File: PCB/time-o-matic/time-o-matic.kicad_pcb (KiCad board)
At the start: 2 copper layers, 1 part, among them U1 ESP32-DevKitC

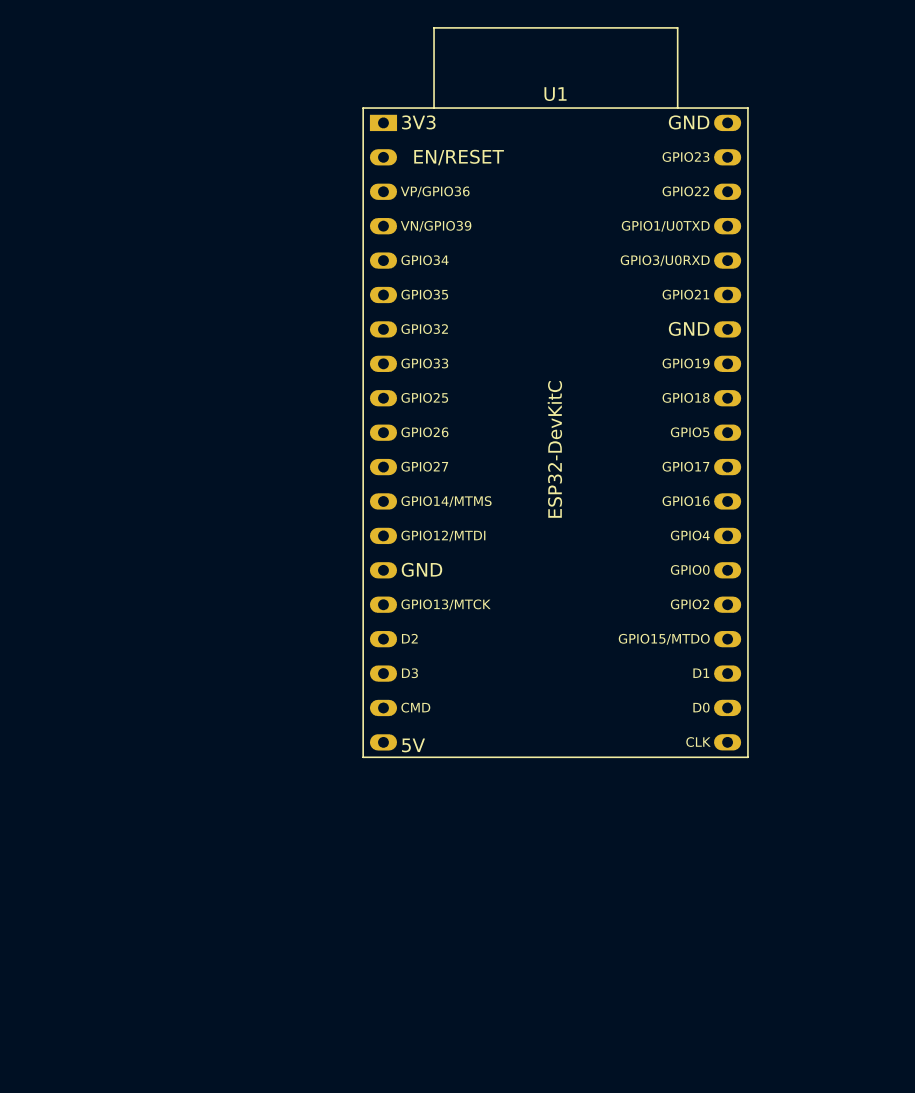
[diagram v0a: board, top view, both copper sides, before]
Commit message: W
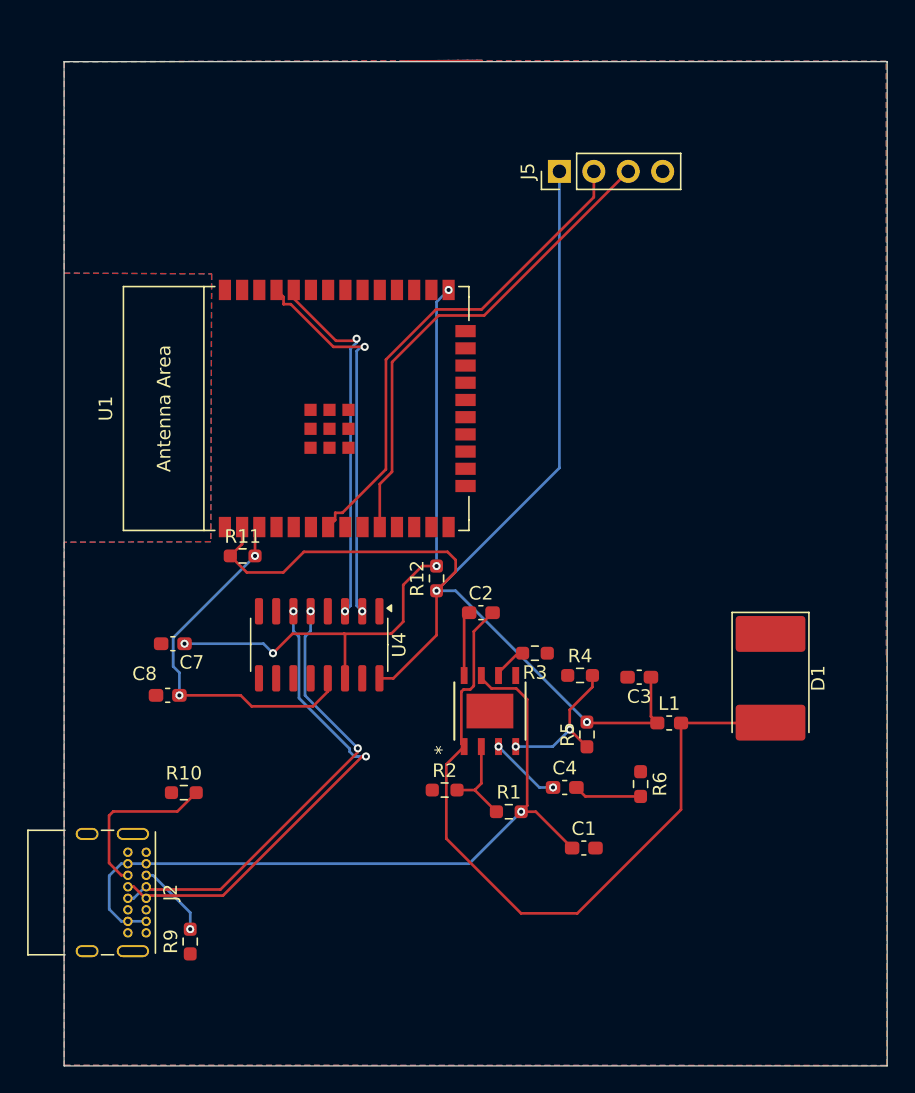
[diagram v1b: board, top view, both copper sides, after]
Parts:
- added C1: 10uF, Capacitor_SMD:C_0603_1608Metric_Pad1.08x0.95mm_HandSolder, F.Cu at (109.6, 106.0)
- added C2: 100nF, Capacitor_SMD:C_0603_1608Metric_Pad1.08x0.95mm_HandSolder, F.Cu at (102.0, 88.6)
- added C3: 22uF, Capacitor_SMD:C_0603_1608Metric_Pad1.08x0.95mm_HandSolder, F.Cu at (113.7, 93.4)
- added C4: 220pF, Capacitor_SMD:C_0603_1608Metric_Pad1.08x0.95mm_HandSolder, F.Cu at (108.2, 101.5)
- added C7: 10uF, Capacitor_SMD:C_0603_1608Metric_Pad1.08x0.95mm_HandSolder, F.Cu at (79.3, 90.9)
- added C8: 10uF, Capacitor_SMD:C_0603_1608Metric_Pad1.08x0.95mm_HandSolder, F.Cu at (78.9, 94.7)
- added D1: D_Schottky, Diode_SMD:D_3220_8050Metric_Pad2.65x5.15mm_HandSolder, F.Cu at (123.4, 93.5)
- added J2: USB_C_Receptacle_USB2.0_14P, Connector_USB:USB_C_Receptacle_GCT_USB4085, F.Cu at (77.3, 106.3)
- added J5: Display Connector, Connector_PinHeader_2.54mm:PinHeader_1x04_P2.54mm_Vertical, F.Cu at (107.8, 56.0)
- added L1: 10uH, Inductor_SMD:L_0603_1608Metric_Pad1.05x0.95mm_HandSolder, F.Cu at (115.9, 96.8)
- added R1: 100k, Resistor_SMD:R_0603_1608Metric_Pad0.98x0.95mm_HandSolder, F.Cu at (104.1, 103.3)
- added R10: 5.1k, Resistor_SMD:R_0603_1608Metric_Pad0.98x0.95mm_HandSolder, F.Cu at (80.1, 101.9)
- added R11: 10k, Resistor_SMD:R_0603_1608Metric_Pad0.98x0.95mm_HandSolder, F.Cu at (84.5, 84.4)
- added R12: 10k, Resistor_SMD:R_0603_1608Metric_Pad0.98x0.95mm_HandSolder, F.Cu at (98.8, 86.1)
- added R2: 24.9k, Resistor_SMD:R_0603_1608Metric_Pad0.98x0.95mm_HandSolder, F.Cu at (99.4, 101.7)
- added R3: 200k, Resistor_SMD:R_0603_1608Metric_Pad0.98x0.95mm_HandSolder, F.Cu at (106.0, 91.6)
- added R4: 40.2k, Resistor_SMD:R_0603_1608Metric_Pad0.98x0.95mm_HandSolder, F.Cu at (109.4, 93.2)
- added R5: 124k, Resistor_SMD:R_0603_1608Metric_Pad0.98x0.95mm_HandSolder, F.Cu at (109.9, 97.6)
- added R6: 68.1k, Resistor_SMD:R_0603_1608Metric_Pad0.98x0.95mm_HandSolder, F.Cu at (113.8, 101.3)
- added R9: 5.1k, Resistor_SMD:R_0603_1608Metric_Pad0.98x0.95mm_HandSolder, F.Cu at (80.6, 112.9)
- added U2: MP1584EN-LF-P, MP1584:SOIC8E_MPS_MNP-L, F.Cu at (102.7, 95.9)
- added U4: CH340C, Package_SO:SOIC-16_3.9x9.9mm_P1.27mm, F.Cu at (90.1, 91.0)
- U1: value ESP32-DevKitC -> ESP32-WROOM-E; footprint PCM_Espressif:ESP32-DevKitC -> PCM_Espressif:ESP32-WROOM-32E
- moved U1 21.6 mm to (90.2, 73.5), turned to 90 degrees
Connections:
- U1 pad 1: unconnected-(U1-3V3-Pad1) -> GND
- U1 pad 10: unconnected-(U1-DAC_2/ADC2_CH9/GPIO26-Pad10) -> i2c-
- U1 pad 14: Net-(U1-GND-Pad14) -> unconnected-(U1-MTDI/GPIO12/ADC2_CH5-Pad14)
- U1 pad 15: unconnected-(U1-MTCK/GPIO13/ADC2_CH4-Pad15) -> GND
- U1 pad 17: unconnected-(U1-SD_DATA3/GPIO10-Pad17) -> (no net)
- U1 pad 18: unconnected-(U1-CMD-Pad18) -> (no net)
- U1 pad 19: unconnected-(U1-5V-Pad19) -> (no net)
- U1 pad 2: unconnected-(U1-CHIP_PU-Pad2) -> +3V3
- U1 pad 20: unconnected-(U1-SD_CLK/GPIO6-Pad20) -> (no net)
- U1 pad 21: unconnected-(U1-SD_DATA0/GPIO7-Pad21) -> (no net)
- U1 pad 22: unconnected-(U1-SD_DATA1/GPIO8-Pad22) -> (no net)
- U1 pad 25: unconnected-(U1-GPIO0/BOOT/ADC2_CH1-Pad25) -> RTS
- U1 pad 3: unconnected-(U1-SENSOR_VP/GPIO36/ADC1_CH0-Pad3) -> DTR
- U1 pad 32: Net-(U1-GND-Pad14) -> (no net)
- U1 pad 34: unconnected-(U1-U0RXD/GPIO3-Pad34) -> P
- U1 pad 35: unconnected-(U1-U0TXD/GPIO1-Pad35) -> N
- U1 pad 38: Net-(U1-GND-Pad14) -> GND
- U1 pad 7: unconnected-(U1-32K_XP/GPIO32/ADC1_CH4-Pad7) -> i2c+
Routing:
- net +3V3: track 0.00 -> 90.7 mm, vias 0 -> 2
- net VIN: track 0.00 -> 55.3 mm, vias 0 -> 1
- net SW: track 0.00 -> 54.1 mm
- net RTS: track 0.00 -> 47.2 mm, vias 0 -> 4
- net i2c+: track 0.00 -> 36.7 mm
- net i2c-: track 0.00 -> 35.8 mm
- net D-: track 0.00 -> 35.7 mm, vias 0 -> 2
- net D+: track 0.00 -> 33.8 mm, vias 0 -> 2
- net N: track 0.00 -> 28.7 mm, vias 0 -> 2
- net DTR: track 0.00 -> 28.0 mm, vias 0 -> 2
- net P: track 0.00 -> 27.1 mm, vias 0 -> 2
- net Net-(J2-CC2): track 0.00 -> 12.4 mm
- net Net-(U2-FB): track 0.00 -> 11.0 mm, vias 0 -> 2
- net EN: track 0.00 -> 6.98 mm
- net Net-(J2-CC1): track 0.00 -> 5.61 mm, vias 0 -> 1
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- added copper zone on B.Cu, net GND
- added copper zone on F.Cu, net GND
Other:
- board outline added: 60.8 x 74.1 mm
